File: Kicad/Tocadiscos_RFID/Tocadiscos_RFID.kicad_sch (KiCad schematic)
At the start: 7 parts, among them M1 Stepper_Motor_unipolar_5pin, P1 Conn_02x20, P2 Conn_02x20, U1 DFPlayer_MiniMP3, U2 ULN2003

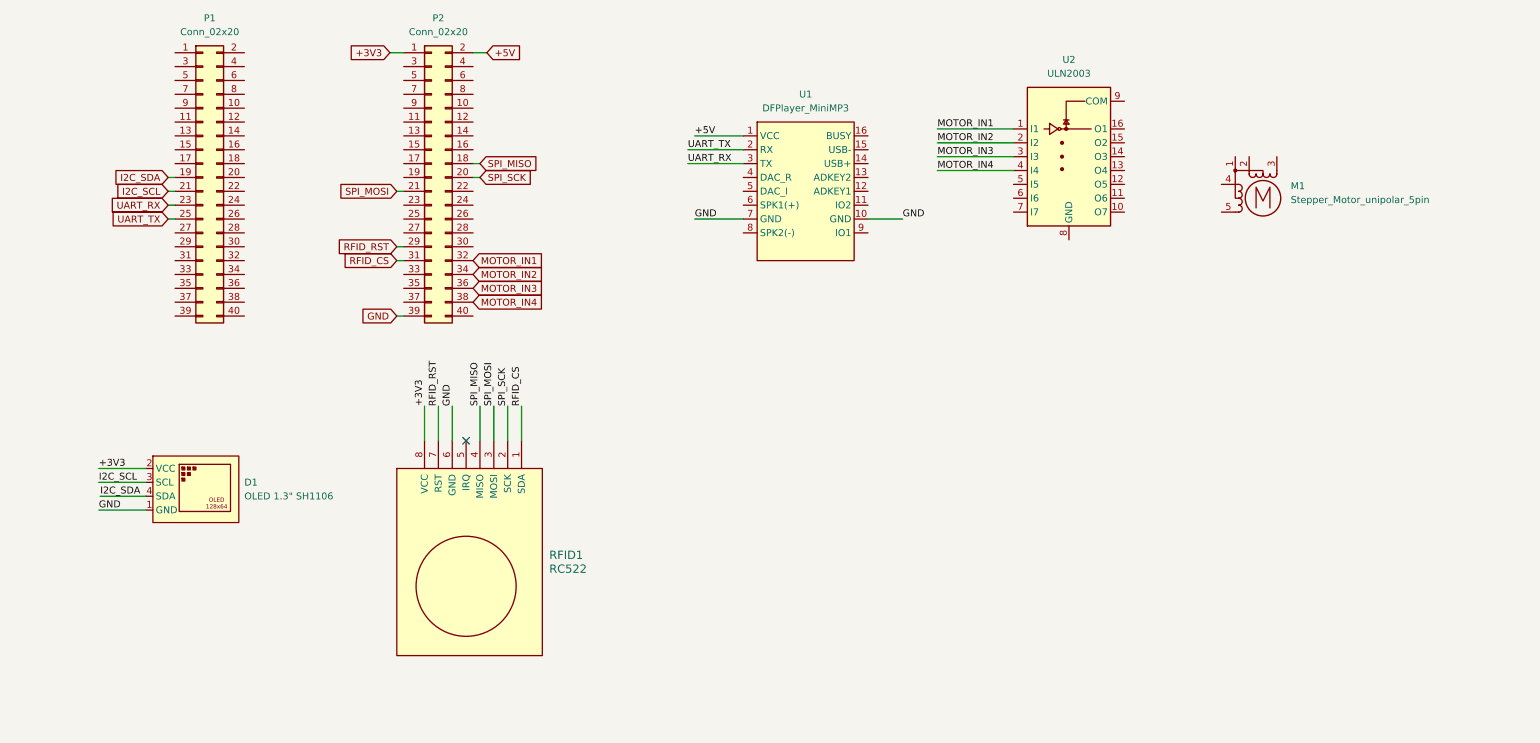
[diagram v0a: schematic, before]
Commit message: .
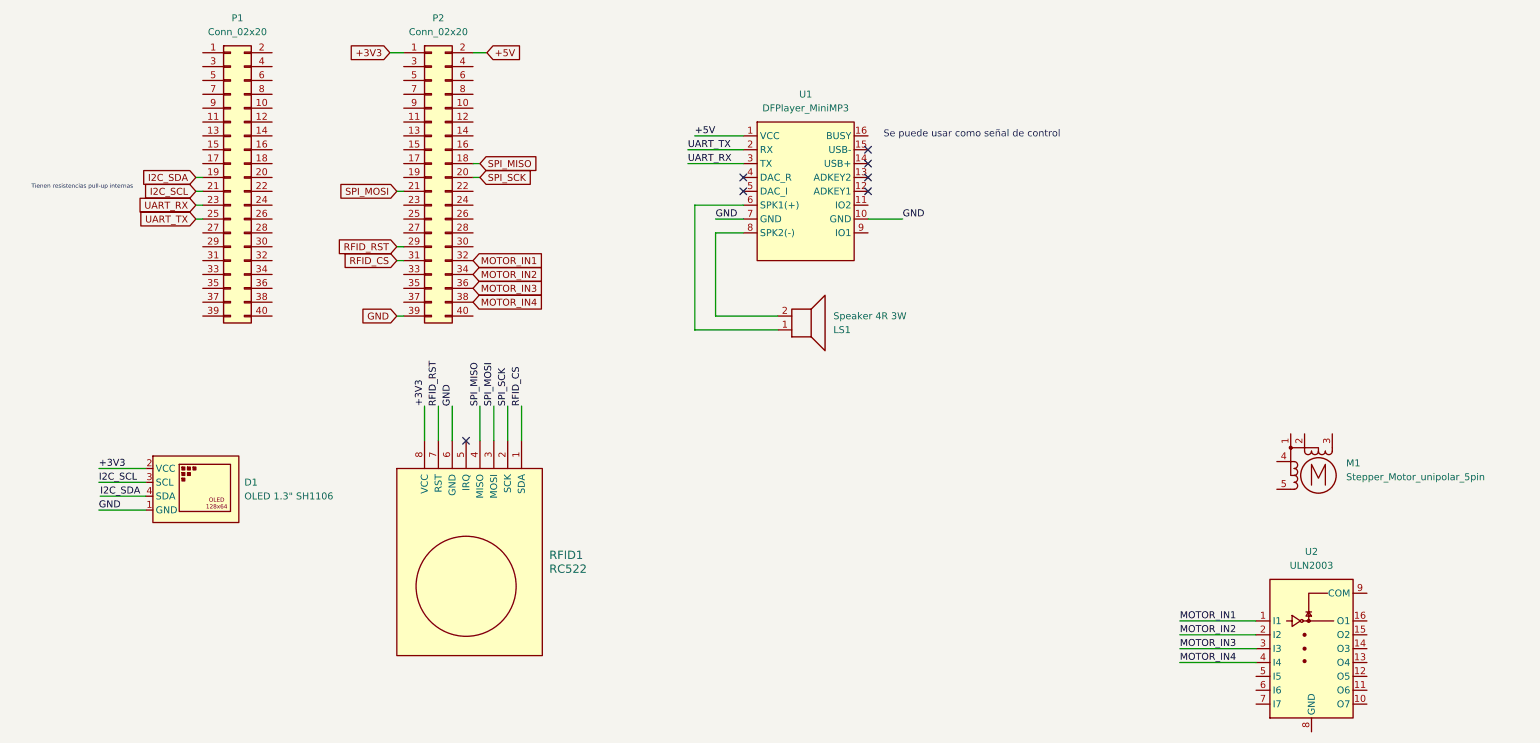
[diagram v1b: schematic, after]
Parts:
- added LS1: Speaker 4R 3W, Package_SON:WSON-8-1EP_6x5mm_P1.27mm_EP3.4x4mm, symbol Device:Speaker
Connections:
- net at U1.6 (SPK1(+)): now also LS1.1
- net at U1.8 (SPK2(-)): now also LS1.2
- no-connect marks 1 -> 7
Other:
- note added: "Se puede usar como señal de control"
- note added: "Tienen resistencias pull-up internas"
- moved on the sheet: M1, P1, U2
